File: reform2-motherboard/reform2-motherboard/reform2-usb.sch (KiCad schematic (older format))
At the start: 90 parts, among them J14 USB_INT2, J17 USB3_A, J5 USB3_A, J6 USB3_A, J9 USB_INT1, U15 TPS2561, U16 TPS2561, U9 TUSB8041, Y1 24MHz

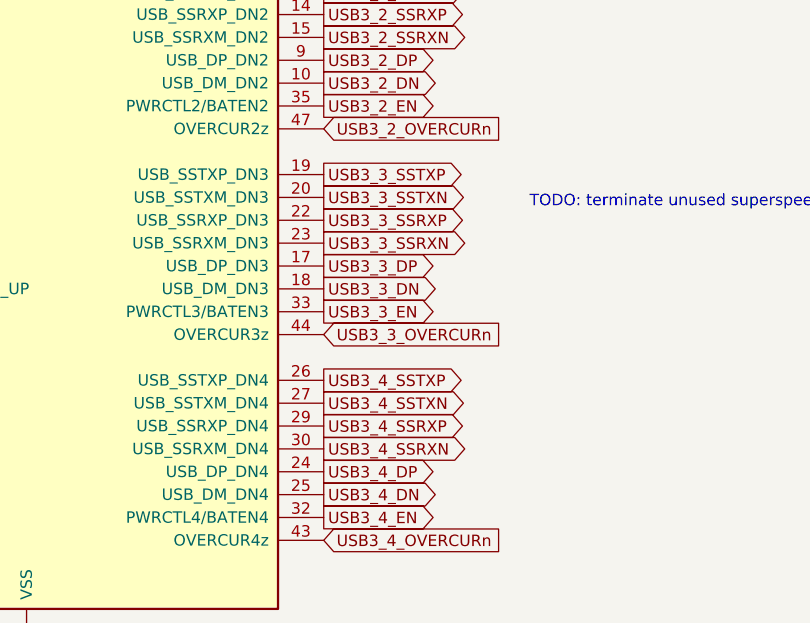
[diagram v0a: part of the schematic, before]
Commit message: reform2: first motherboard fully routed, checks TBD
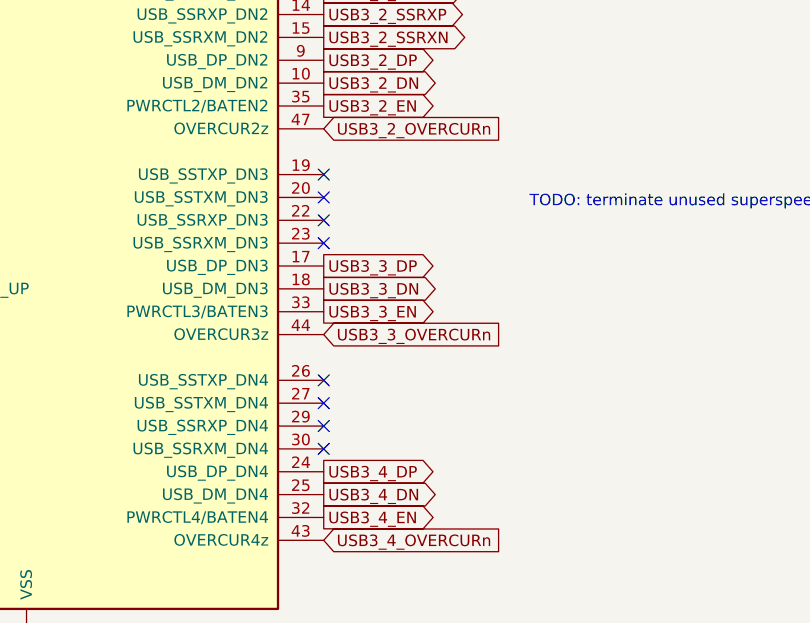
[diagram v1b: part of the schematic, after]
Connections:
- net USB3_3_SSRXN: no longer names the net of U9.23 (USB_SSRXM_DN3)
- net USB3_3_SSRXP: no longer names the net of U9.22 (USB_SSRXP_DN3)
- net USB3_3_SSTXN: no longer names the net of U9.20 (USB_SSTXM_DN3)
- net USB3_3_SSTXP: no longer names the net of U9.19 (USB_SSTXP_DN3)
- net USB3_4_SSRXN: no longer names the net of U9.30 (USB_SSRXM_DN4)
- net USB3_4_SSRXP: no longer names the net of U9.29 (USB_SSRXP_DN4)
- net USB3_4_SSTXN: no longer names the net of U9.27 (USB_SSTXM_DN4)
- net USB3_4_SSTXP: no longer names the net of U9.26 (USB_SSTXP_DN4)
- no-connect marks 3 -> 11
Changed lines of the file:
@@
 Text GLabel 13500 4200 2    50   Output ~ 0
 USB3_2_DN
-Text GLabel 13500 4600 2    50   Output ~ 0
-USB3_3_SSTXP
-Text GLabel 13500 4700 2    50   Output ~ 0
-USB3_3_SSTXN
-Text GLabel 13500 4800 2    50   Output ~ 0
-USB3_3_SSRXP
-Text GLabel 13500 4900 2    50   Output ~ 0
-USB3_3_SSRXN
 Text GLabel 13500 5000 2    50   Output ~ 0
 USB3_3_DP
 Text GLabel 13500 5100 2    50   Output ~ 0
 USB3_3_DN
-Text GLabel 13500 5500 2    50   Output ~ 0
-USB3_4_SSTXP
-Text GLabel 13500 5600 2    50   Output ~ 0
-USB3_4_SSTXN
-Text GLabel 13500 5700 2    50   Output ~ 0
-USB3_4_SSRXP
-Text GLabel 13500 5800 2    50   Output ~ 0
-USB3_4_SSRXN
 Text GLabel 13500 5900 2    50   Output ~ 0
 USB3_4_DP
@@
 Text Notes 14400 4750 0    50   ~ 0
 TODO: terminate unused superspeeds?
+NoConn ~ 13500 4600
+NoConn ~ 13500 4700
+NoConn ~ 13500 4800
+NoConn ~ 13500 4900
+NoConn ~ 13500 5500
+NoConn ~ 13500 5600
+NoConn ~ 13500 5700
+NoConn ~ 13500 5800
 $EndSCHEMATC
